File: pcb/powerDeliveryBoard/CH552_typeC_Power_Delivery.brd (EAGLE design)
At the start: 35.6 x 12 mm, 14 parts, among them J4 USB_A_SMT_MALE, U2 CH552G

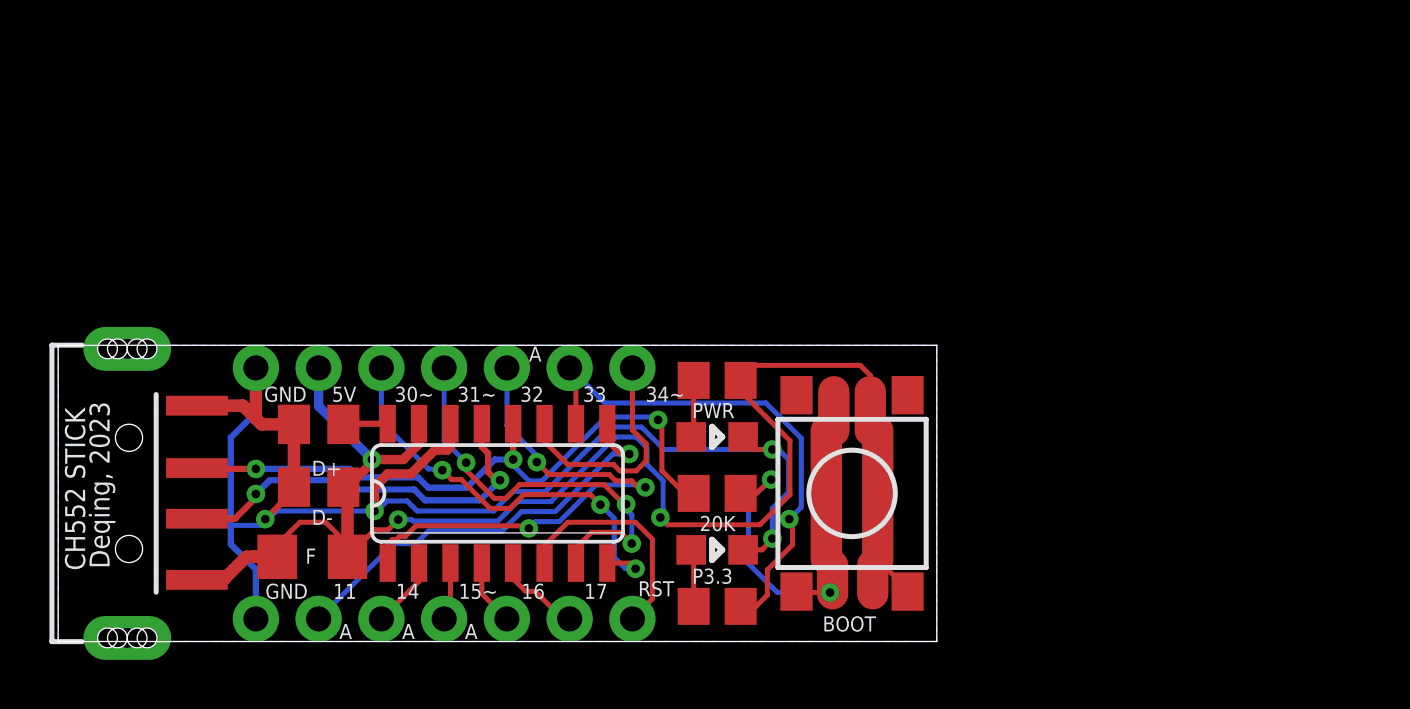
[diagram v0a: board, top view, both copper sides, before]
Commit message: make some progress
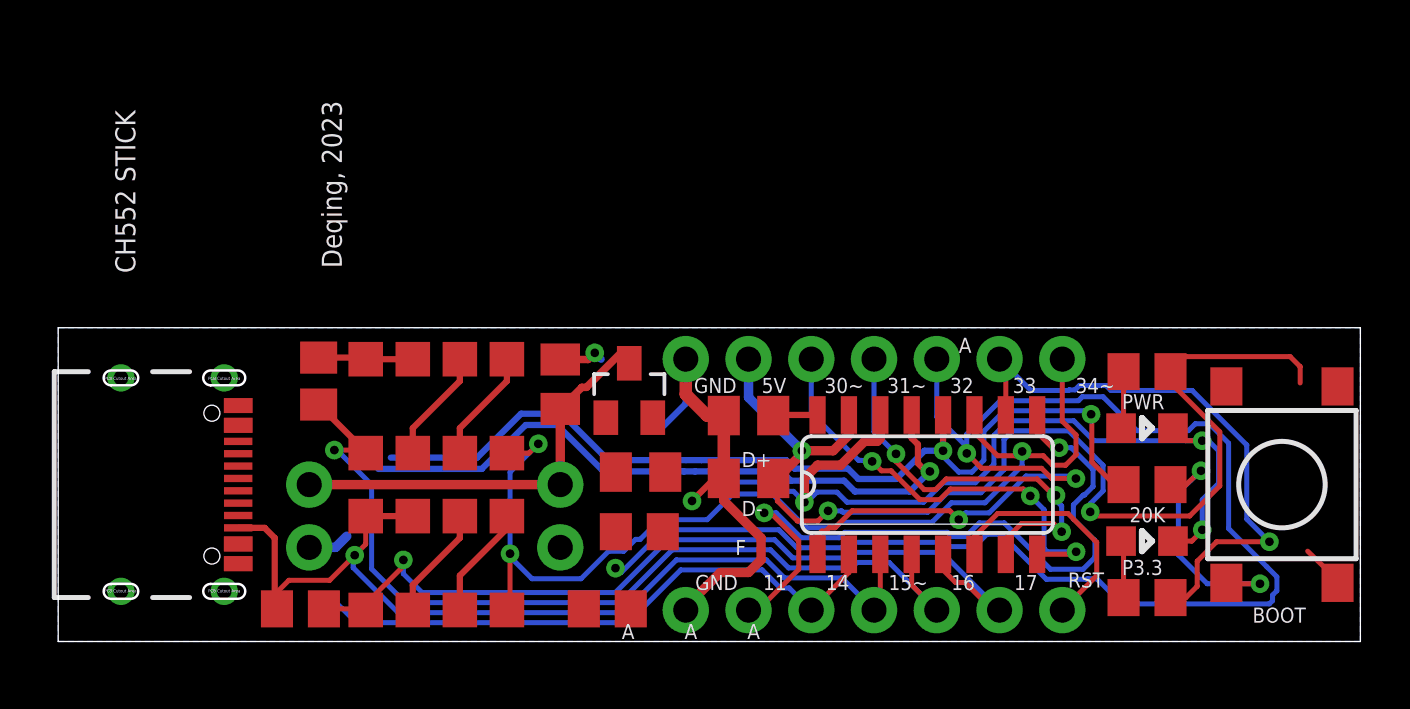
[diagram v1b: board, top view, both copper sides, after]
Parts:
- removed F1: (no value), adafruit:R1206
- added C3, C4: 0.1uF, rcl:C0805K
- added D1, D2, D3, D4, D5, D6, D7, D8: (no value), diode:SOD123
- added J3: 629722000214, Wurth_Connectors_WR-USB:629722000214
- added J5: (no value), SparkFun-Connectors:1X02_NO_SILK
- added R4: 14.7K, rcl:R0805
- added R5: 2K, rcl:R0805
- added R6, R7: 1K, rcl:R0805
- added U1: MCP1703CB, linear:SOT23
- J4: value USB_A_SMT_MALE -> (none); device SparkFun-Connectors:USB-A-SMT-MALE -> SparkFun-Connectors:1X02_NO_SILK
- moved C1 17.4 mm to (27.9, 6.60)
- moved C2 17.4 mm to (27.9, 9.14)
- moved GOLD_ORB_SM1 17.4 mm to (47.5, 7.72)
- moved J1 17.4 mm to (25.4, 1.27)
- moved J2 17.4 mm to (25.4, 11.4)
- moved LED1 17.4 mm to (44.1, 8.64)
- moved LED2 17.4 mm to (44.1, 4.06)
- moved R1 17.4 mm to (44.1, 6.35)
- moved R2 17.4 mm to (44.1, 10.9)
- moved R3 17.4 mm to (44.1, 1.78)
- moved S1 17.4 mm to (49.5, 6.35)
- moved U2 17.4 mm to (35.2, 6.35)
- moved J4 15.6 mm to (10.2, 3.81), turned to 90 degrees
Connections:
- new net N$4: D2.C, D3.A
- new net N$5: D3.C, D4.A
- new net N$6: D5.C, D7.A
- new net N$7: D7.C, D8.A
- new net VUSB: C3.1, J3.A4, J3.A9, J3.B4, J3.B9, J4.2, J5.2, U1.3
- net +5V: now also C4.1, R4.1, U1.2; no longer F1.1, F1.2, J4.VBUS1
- net GND: now also C3.2, C4.2, J3.A1, J3.A12, J3.B1, J3.B12, J4.1, J5.1, R5.2, U1.1; no longer J4.GND1
- net P1.4: now also D1.A, D2.A, J3.A5, R6.2
- net P1.5: now also D5.A, D6.A, J3.B5, R7.2
- net P1.6: now also D1.C, R6.1
- net P1.7: now also D6.C, R7.1
- net P3.2: now also R4.2, R5.1
- net P3.4: now also D4.C, D8.C
- net USB_D+: now also J3.A6, J3.B6; no longer J4.D+1
- net USB_D-: now also J3.A7, J3.B7; no longer J4.D-1
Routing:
- net P3.2: track 21.5 -> 71.4 mm, vias 3 -> 4
- net P1.5: track 2.37 -> 38.6 mm, vias 0 -> 1
- net P1.6: track 2.68 -> 37.8 mm, vias 0 -> 1
- net P3.4: track 9.48 -> 43.6 mm, vias 0 -> 3
- net P1.7: track 3.59 -> 35.2 mm, vias 0 -> 1
- net P1.4: track 2.89 -> 27.8 mm
- net +5V: track 66.7 -> 48.3 mm
- net VUSB: track 0.00 -> 16.7 mm
- net USB_D+: track 26.3 -> 38.0 mm, vias 3 -> 2
- net P1.1: track 17.2 -> 28.8 mm, vias 1 -> 2
- net USB_D-: track 16.4 -> 27.2 mm, vias 2 -> 1
- net N$1: track 19.1 -> 10.5 mm
- net N$5: track 0.00 -> 4.59 mm
- net N$7: track 0.00 -> 4.59 mm
- net N$6: track 0.00 -> 4.59 mm
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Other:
- board size 35.6 x 12 mm -> 52.7 x 12.7 mm
